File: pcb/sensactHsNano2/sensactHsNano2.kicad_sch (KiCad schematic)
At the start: 55 parts, among them J1 HMI, J2 SensactBusConnector, J3 CAN+485, J5 Audio, J6 Conn_01x03, J8 Conn_01x10, J9 24V, SW1 TERM ON, SW2 OFF TERM ON, SW3 Reset, SW4 PROG_PWR, U10 INA219AxD, U11 L78L15_SOT89, U3 ESP32, U4 DS2482, U5 SN65HVD230, U6 MAX3485, U8 LM358, U9 MCP4728

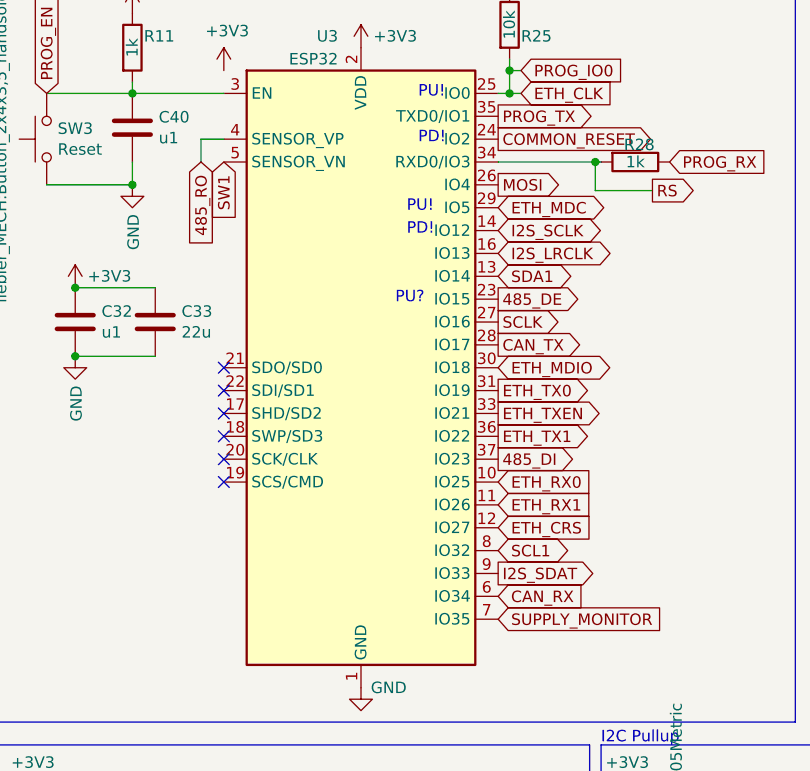
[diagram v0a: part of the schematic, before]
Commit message: Various
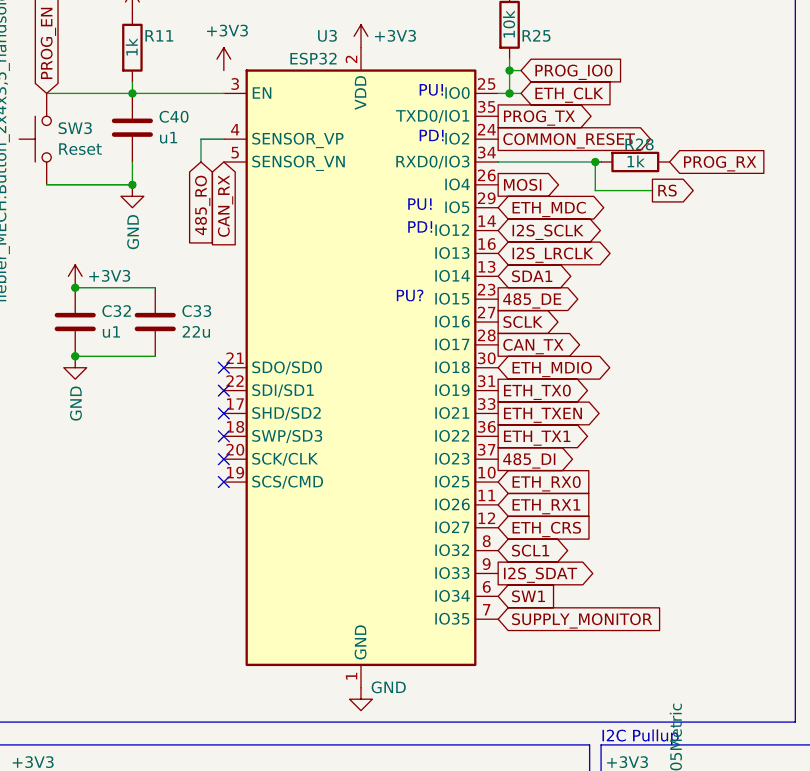
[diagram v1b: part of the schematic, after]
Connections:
- net CAN_RX: now also U3.5 (SENSOR_VN); no longer U3.6 (IO34)
- net SW1: now also U3.6 (IO34); no longer U3.5 (SENSOR_VN)
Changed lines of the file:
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@@
     )
   )
-  (global_label "CAN_RX" (shape input) (at 74.93 86.36 0) (fields_autoplaced)
-    (effects (font (size 1.27 1.27)) (justify left))
-    (property "Intersheet References" "${INTERSHEET_REFS}" (id 0) (at 0 -2.54 0)
+  (global_label "CAN_RX" (shape input) (at 44.45 38.1 270) (fields_autoplaced)
+    (effects (font (size 1.27 1.27)) (justify right))
+    (property "Intersheet References" "${INTERSHEET_REFS}" (id 0) (at 133.35 -36.83 0)
       (effects (font (size 1.27 1.27)) hide)
     )
@@
     )
   )
-  (global_label "SW1" (shape input) (at 44.45 38.1 270) (fields_autoplaced)
-    (effects (font (size 1.27 1.27)) (justify right))
-    (property "Intersheet References" "${INTERSHEET_REFS}" (id 0) (at 44.3706 44.2947 90)
-      (effects (font (size 1.27 1.27)) (justify right) hide)
+  (global_label "SW1" (shape input) (at 74.93 86.36 0) (fields_autoplaced)
+    (effects (font (size 1.27 1.27)) (justify left))
+    (property "Intersheet References" "${INTERSHEET_REFS}" (id 0) (at 81.1247 86.4394 0)
+      (effects (font (size 1.27 1.27)) (justify left) hide)
     )
   )
@@
       (reference "#PWR012") (unit 1) (value "GND") (footprint "")
     )
-    (path "/00000000-0000-0000-0000-000060e30b7a/00000000-0000-0000-0000-00005e10cb5e"
+    (path "/00000000-0000-0000-0000-00006181a2e2/3a9196e9-edcd-4f47-bb3f-07f82e25dbdc"
       (reference "#PWR013") (unit 1) (value "GND") (footprint "")
     )
@@
       (reference "#PWR014") (unit 1) (value "+3V3") (footprint "")
     )
-    (path "/00000000-0000-0000-0000-000060e30b7a/00000000-0000-0000-0000-00005e0b73e9"
-      (reference "#PWR015") (unit 1) (value "GND") (footprint "")
-    )
     (path "/00000000-0000-0000-0000-000060e30b7a/00000000-0000-0000-0000-00005e0dad05"
       (reference "#PWR016") (unit 1) (value "GND") (footprint "")
@@
       (reference "#PWR025") (unit 1) (value "GND") (footprint "")
     )
-    (path "/00000000-0000-0000-0000-000060e30b7a/00000000-0000-0000-0000-00005e10d619"
-      (reference "#PWR026") (unit 1) (value "GND") (footprint "")
-    )
     (path "/00000000-0000-0000-0000-000060e5a575"
       (reference "#PWR027") (unit 1) (value "+3V3") (footprint "")
@@
       (reference "#PWR0151") (unit 1) (value "+3V3") (footprint "")
     )
+    (path "/00000000-0000-0000-0000-000060e30b7a/e7cb7bc1-2d67-4af7-b28d-d561be0de79a"
+      (reference "#PWR0152") (unit 1) (value "GND") (footprint "")
+    )
     (path "/00000000-0000-0000-0000-00005f9c3c99/00000000-0000-0000-0000-00005f9dd337"
       (reference "C1") (unit 1) (value "470u") (footprint "Capacitor_THT:CP_Radial_D10.0mm_P3.50mm")
@@
     )
     (path "/00000000-0000-0000-0000-000060e30b7a/00000000-0000-0000-0000-00005e109cd1"
-      (reference "C21") (unit 1) (value "u1") (footprint "Capacitor_SMD:C_0805_2012Metric_Pad1.18x1.45mm_HandSolder")
+      (reference "C21") (unit 1) (value "u1") (footprint "Capacitor_SMD:C_0402_1005Metric")
     )
     (path "/00000000-0000-0000-0000-00005fa43ad6"
@@
     )
     (path "/00000000-0000-0000-0000-00006181a2e2/eb914753-4ad8-44fc-93fd-14f530d0ab5b"
-      (reference "J7") (unit 1) (value "PROG") (footprint "liebler_CONN:USB_C_Receptacle_HRO_TYPE-C-31-M-12_IMPROVED")
+      (reference "J7") (unit 1) (value "PROG") (footprint "liebler_CONN:USB_C_Receptacle_HRO_TYPE-C-31-M-12_smaller")
     )
     (path "/00000000-0000-0000-0000-000061938435"
@@
       (reference "NT1") (unit 1) (value "Net-Tie_2") (footprint "NetTie:NetTie-2_SMD_Pad2.0mm")
     )
+    (path "/00000000-0000-0000-0000-000060e30b7a/c83ee589-2a8a-4166-bee2-d2f600b8d91e"
+      (reference "NT2") (unit 1) (value "NetTie_2") (footprint "NetTie:NetTie-2_SMD_Pad0.5mm")
+    )
     (path "/00000000-0000-0000-0000-00006181a2e2/dd64bd92-873a-41e2-947c-df9be8b62d94"
-      (reference "Q1") (unit 1) (value "BC817") (footprint "Package_TO_SOT_SMD:SOT-23")
+      (reference "Q1") (unit 1) (value "BC817") (footprint "liebler_SEMICONDUCTORS:SOT-23_smaller")
     )
     (path "/00000000-0000-0000-0000-00006181a2e2/32659d89-6784-4859-9fd1-5b6349b2ee2a"
-      (reference "Q2") (unit 1) (value "BC817") (footprint "Package_TO_SOT_SMD:SOT-23")
+      (reference "Q2") (unit 1) (value "BC817") (footprint "liebler_SEMICONDUCTORS:SOT-23_smaller")
     )
     (path "/00000000-0000-0000-0000-00005fa49518"
@@
     )
     (path "/00000000-0000-0000-0000-00005f9c3c99/00000000-0000-0000-0000-000061306266"
-      (reference "U1") (unit 1) (value "TAS5805M") (footprint "liebler_SEMICONDUCTORS:TSSOP-28_4.4x9.7mm_Pitch0.65mm_pad_handsolder")
+      (reference "U1") (unit 1) (value "TAS5805M") (footprint "Package_SO:HTSSOP-28-1EP_4.4x9.7mm_P0.65mm_EP2.85x5.4mm_ThermalVias")
     )
     (path "/00000000-0000-0000-0000-000060e30b7a/00000000-0000-0000-0000-00006124e6ff"
@@
       (reference "U11") (unit 1) (value "L78L15_SOT89") (footprint "Package_TO_SOT_SMD:SOT-89-3_Handsoldering")
     )
-    (path "/00000000-0000-0000-0000-00006181a2e2/f00e656c-e83a-4766-909c-2e0d3eea4f0e"
-      (reference "U13") (unit 1) (value "CH340C") (footprint "Package_SO:SOIC-16_3.9x9.9mm_P1.27mm")
+    (path "/00000000-0000-0000-0000-00006181a2e2/e46ba44c-f9ee-428c-a18c-f36ebf366e7e"
+      (reference "U12") (unit 1) (value "CH340K") (footprint "liebler_SEMICONDUCTORS:SSOP-10_3.9x4.9mm_P1.00mm_EP")
     )
     (path "/00000000-0000-0000-0000-000060e30b7a/00000000-0000-0000-0000-00005e0b1bef"
-      (reference "X1") (unit 1) (value "50MHz") (footprint "Oscillator:Oscillator_SMD_EuroQuartz_XO32-4Pin_3.2x2.5mm_HandSoldering")
-    )
-  )
+      (reference "X1") (unit 1) (value "50MHz") (footprint "Oscillator:Oscillator_SMD_SeikoEpson_SG8002CE-4Pin_3.2x2.5mm")
+    )
+  )
